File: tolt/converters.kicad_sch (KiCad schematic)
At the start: 60 parts, among them J11 Conn_01x05, U14 AMS1117-3.3, U15 LP5907MFX-3.3, U16 TPS62173DSG, U24 LTC7138xMSE, U25 LNK306D

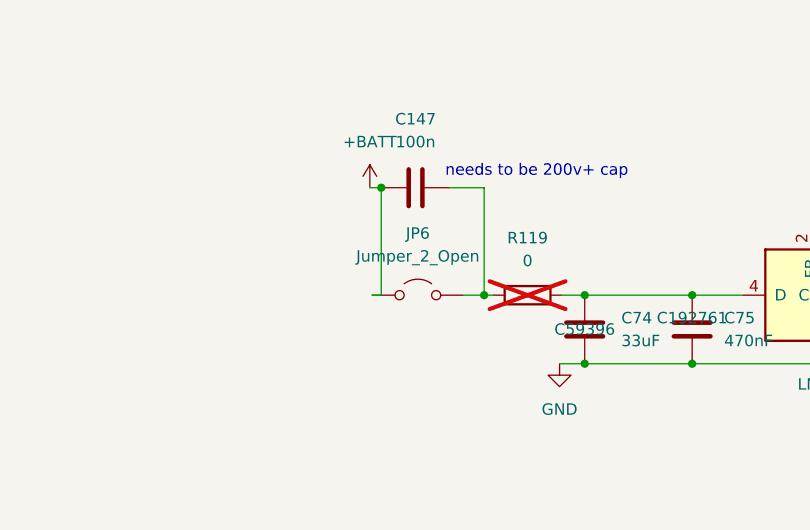
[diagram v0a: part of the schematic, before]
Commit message: 12vdc
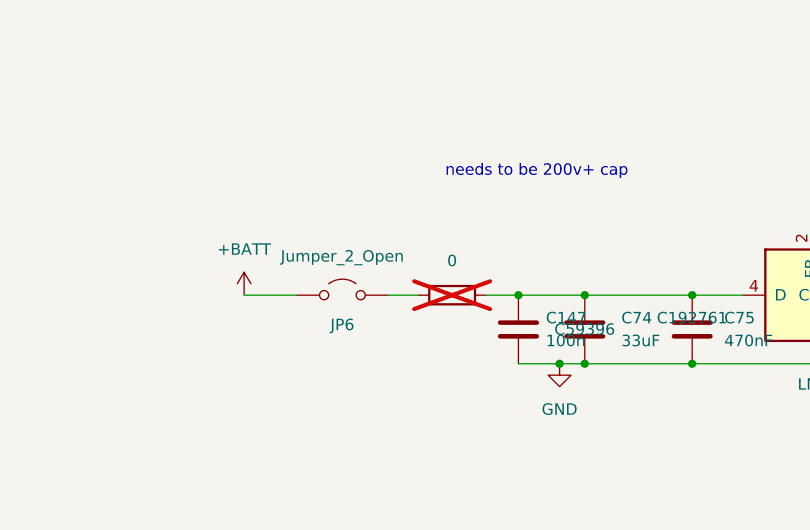
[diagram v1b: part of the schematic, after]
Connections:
- net +BATT: no longer C147.1
- net GND: now also C147.2
- net at JP6.2 (B), R119.1: no longer C147.2
- net at C74.1, C75.1, R119.2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: now also C147.1
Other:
- moved on the sheet: C147, JP6
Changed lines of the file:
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@@
 	)
 	(junction
-		(at 200.152 42.418)
+		(at 157.48 96.52)
 		(diameter 0)
 		(color 0 0 0 0)
 	)
 	(junction
-		(at 157.48 96.52)
+		(at 63.754 106.426)
 		(diameter 0)
 		(color 0 0 0 0)
 	)
 	(junction
-		(at 63.754 106.426)
+		(at 315.722 54.356)
 		(diameter 0)
 		(color 0 0 0 0)
 	)
 	(junction
-		(at 315.722 54.356)
+		(at 215.392 54.356)
 		(diameter 0)
 		(color 0 0 0 0)
@@
 	)
 	(junction
+		(at 219.964 61.976)
+		(diameter 0)
+		(color 0 0 0 0)
+	)
+	(junction
 		(at 338.328 199.644)
 		(diameter 0)
@@
 	)
 	(junction
-		(at 211.582 54.356)
-		(diameter 0)
-		(color 0 0 0 0)
-	)
-	(junction
 		(at 112.268 48.514)
 		(diameter 0)
@@
 	(wire
 		(pts
-			(xy 200.152 42.418) (xy 200.152 54.356)
-		)
-		(stroke
-			(width 0)
-			(type default)
-		)
-	)
-	(wire
-		(pts
 			(xy 169.926 96.52) (xy 179.07 96.52)
 		)
@@
 	(wire
 		(pts
-			(xy 211.582 54.356) (xy 212.598 54.356)
-		)
-		(stroke
-			(width 0)
-			(type default)
-		)
-	)
-	(wire
-		(pts
 			(xy 60.96 163.576) (xy 60.96 181.61)
 		)
@@
 	(wire
 		(pts
-			(xy 211.582 54.356) (xy 209.296 54.356)
-		)
-		(stroke
-			(width 0)
-			(type default)
-		)
-	)
-	(wire
-		(pts
-			(xy 200.152 54.356) (xy 199.136 54.356)
+			(xy 200.914 54.356) (xy 204.216 54.356)
 		)
 		(stroke
@@
 	(wire
 		(pts
-			(xy 220.218 54.356) (xy 222.758 54.356)
+			(xy 286.004 52.832) (xy 286.004 54.356)
 		)
 		(stroke
@@
 	(wire
 		(pts
-			(xy 286.004 52.832) (xy 286.004 54.356)
+			(xy 211.836 54.356) (xy 215.392 54.356)
 		)
 		(stroke
@@
 	(wire
 		(pts
-			(xy 198.882 42.418) (xy 200.152 42.418)
-		)
-		(stroke
-			(width 0)
-			(type default)
-		)
-	)
-	(wire
-		(pts
 			(xy 275.844 54.356) (xy 264.922 54.356)
 		)
@@
 	(wire
 		(pts
+			(xy 215.392 61.976) (xy 219.964 61.976)
+		)
+		(stroke
+			(width 0)
+			(type default)
+		)
+	)
+	(wire
+		(pts
 			(xy 160.274 161.036) (xy 148.844 161.036)
 		)
@@
 	(wire
 		(pts
-			(xy 207.772 42.418) (xy 211.582 42.418)
+			(xy 215.392 54.356) (xy 222.758 54.356)
 		)
 		(stroke
@@
 	(wire
 		(pts
-			(xy 211.582 42.418) (xy 211.582 54.356)
+			(xy 184.912 54.356) (xy 190.754 54.356)
 		)
 		(stroke
@@
 	(symbol
 		(lib_id "Device:R")
-		(at 216.408 54.356 90)
+		(at 208.026 54.356 90)
 		(unit 1)
 		(exclude_from_sim no)
@@
 		(on_board yes)
 		(dnp yes)
-		(fields_autoplaced yes)
 		(property "Reference" "R119"
-			(at 216.408 48.006 90)
+			(at 194.31 45.974 90)
 			(effects
 				(font
 					(size 1.27 1.27)
 				)
+				(hide yes)
 			)
 		)
 		(property "Value" "0"
-			(at 216.408 50.546 90)
+			(at 208.026 50.546 90)
 			(effects
 				(font
@@
 		)
 		(property "Footprint" "Resistor_SMD:R_0603_1608Metric"
-			(at 216.408 56.134 90)
+			(at 208.026 56.134 90)
 			(effects
 				(font
@@
 		)
 		(property "Datasheet" "~"
-			(at 216.408 54.356 0)
+			(at 208.026 54.356 0)
 			(effects
 				(font
@@
 		)
 		(property "Description" "Resistor"
-			(at 216.408 54.356 0)
+			(at 208.026 54.356 0)
 			(effects
 				(font
@@
 		)
 		(property "Availability" ""
-			(at 216.408 54.356 0)
+			(at 208.026 54.356 0)
 			(effects
 				(font
@@
 		)
 		(property "Check_prices" ""
-			(at 216.408 54.356 0)
+			(at 208.026 54.356 0)
 			(effects
 				(font
@@
 		)
 		(property "Description_1" ""
-			(at 216.408 54.356 0)
+			(at 208.026 54.356 0)
 			(effects
 				(font
@@
 		)
 		(property "MANUFACTURER" ""
-			(at 216.408 54.356 0)
+			(at 208.026 54.356 0)
 			(effects
 				(font
@@
 		)
 		(property "MAXIMUM_PACKAGE_HEIGHT" ""
-			(at 216.408 54.356 0)
+			(at 208.026 54.356 0)
 			(effects
 				(font
@@
 		)
 		(property "MF" ""
-			(at 216.408 54.356 0)
+			(at 208.026 54.356 0)
 			(effects
 				(font
@@
 		)
 		(property "MFR PT" ""
-			(at 216.408 54.356 0)
+			(at 208.026 54.356 0)
 			(effects
 				(font
@@
 		)
 		(property "MP" ""
-			(at 216.408 54.356 0)
+			(at 208.026 54.356 0)
 			(effects
 				(font
@@
 		)
 		(property "PARTREV" ""
-			(at 216.408 54.356 0)
+			(at 208.026 54.356 0)
 			(effects
 				(font
@@
 		)
 		(property "Package" ""
-			(at 216.408 54.356 0)
+			(at 208.026 54.356 0)
 			(effects
 				(font
@@
 		)
 		(property "Price" ""
-			(at 216.408 54.356 0)
+			(at 208.026 54.356 0)
 			(effects
 				(font
@@
 		)
 		(property "STANDARD" ""
-			(at 216.408 54.356 0)
+			(at 208.026 54.356 0)
 			(effects
 				(font
@@
 		)
 		(property "SnapEDA_Link" ""
-			(at 216.408 54.356 0)
+			(at 208.026 54.356 0)
 			(effects
 				(font
@@
 	(symbol
 		(lib_id "power:+BATT")
-		(at 198.882 42.418 0)
+		(at 184.912 54.356 0)
 		(unit 1)
 		(exclude_from_sim no)
@@
 		(fields_autoplaced yes)
 		(property "Reference" "#PWR0164"
-			(at 198.882 46.228 0)
+			(at 184.912 58.166 0)
 			(effects
 				(font
@@
 		)
 		(property "Value" "+BATT"
-			(at 198.882 37.338 0)
+			(at 184.912 49.276 0)
 			(effects
 				(font
@@
 		)
 		(property "Footprint" ""
-			(at 198.882 42.418 0)
+			(at 184.912 54.356 0)
 			(effects
 				(font
@@
 		)
 		(property "Datasheet" ""
-			(at 198.882 42.418 0)
+			(at 184.912 54.356 0)
 			(effects
 				(font
@@
 		)
 		(property "Description" "Power symbol creates a global label with name \"+BATT\""
-			(at 198.882 42.418 0)
+			(at 184.912 54.356 0)
 			(effects
 				(font
@@
 	(symbol
 		(lib_id "Device:C")
-		(at 203.962 42.418 90)
+		(at 215.392 58.166 0)
 		(unit 1)
 		(exclude_from_sim no)
@@
 		(fields_autoplaced yes)
 		(property "Reference" "C147"
-			(at 203.962 34.798 90)
+			(at 218.44 56.8959 0)
 			(effects
 				(font
 					(size 1.27 1.27)
 				)
+				(justify left)
 			)
 		)
 		(property "Value" "100n"
-			(at 203.962 37.338 90)
+			(at 218.44 59.4359 0)
 			(effects
 				(font
 					(size 1.27 1.27)
 				)
+				(justify left)
 			)
 		)
 		(property "Footprint" "Capacitor_SMD:C_1210_3225Metric"
-			(at 207.772 41.4528 0)
+			(at 216.3572 61.976 0)
 			(effects
 				(font
@@
 		)
 		(property "Datasheet" "~"
-			(at 203.962 42.418 0)
+			(at 215.392 58.166 0)
 			(effects
 				(font
@@
 		)
 		(property "Description" "Unpolarized capacitor"
-			(at 203.962 42.418 0)
+			(at 215.392 58.166 0)
 			(effects
 				(font
@@
 	(symbol
 		(lib_id "Jumper:Jumper_2_Open")
-		(at 204.216 54.356 0)
+		(at 195.834 54.356 0)
 		(unit 1)
 		(exclude_from_sim yes)
@@
 		(on_board yes)
 		(dnp no)
-		(fields_autoplaced yes)
 		(property "Reference" "JP6"
-			(at 204.216 47.498 0)
+			(at 195.834 57.658 0)
 			(effects
 				(font
@@
 		)
 		(property "Value" "Jumper_2_Open"
-			(at 204.216 50.038 0)
+			(at 195.834 50.038 0)
 			(effects
 				(font
@@
 		)
 		(property "Footprint" "Connector_PinHeader_2.54mm:PinHeader_1x02_P2.54mm_Vertical"
-			(at 204.216 54.356 0)
+			(at 195.834 54.356 0)
 			(effects
 				(font
@@
 		)
 		(property "Datasheet" "~"
-			(at 204.216 54.356 0)
+			(at 195.834 54.356 0)
 			(effects
 				(font
@@
 		)
 		(property "Description" "Jumper, 2-pole, open"
-			(at 204.216 54.356 0)
+			(at 195.834 54.356 0)
 			(effects
 				(font

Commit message: begenning of lcsc part assign
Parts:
- C102, C105: footprint Capacitor_SMD:C_2220_5750Metric_Pad1.97x5.40mm_HandSolder -> Capacitor_SMD:C_2220_5750Metric
- C149, C71, C73, C85: LCSC (none) -> C138687
- C150: footprint Capacitor_SMD:C_1206_3216Metric_Pad1.33x1.80mm_HandSolder -> Capacitor_SMD:C_1206_3216Metric
- C66: LCSC (none) -> C15008
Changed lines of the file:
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@@
 			)
 		)
+		(property "LCSC" "C138687"
+			(at 170.942 164.846 0)
+			(effects
+				(font
+					(size 1.27 1.27)
+				)
+				(hide yes)
+			)
+		)
 		(pin "1"
 		)
@@
 			)
 		)
+		(property "LCSC" "C138687"
+			(at 112.268 44.704 0)
+			(effects
+				(font
+					(size 1.27 1.27)
+				)
+				(hide yes)
+			)
+		)
 		(pin "1"
 		)
@@
 			)
 		)
+		(property "LCSC" "C138687"
+			(at 148.844 164.846 0)
+			(effects
+				(font
+					(size 1.27 1.27)
+				)
+				(hide yes)
+			)
+		)
 		(pin "1"
 		)
@@
 			)
 		)
+		(property "LCSC" "C138687"
+			(at 47.752 43.688 0)
+			(effects
+				(font
+					(size 1.27 1.27)
+				)
+				(hide yes)
+			)
+		)
 		(pin "1"
 		)
@@
 			)
 		)
-		(property "Footprint" "Capacitor_SMD:C_2220_5750Metric_Pad1.97x5.40mm_HandSolder"
+		(property "Footprint" "Capacitor_SMD:C_2220_5750Metric"
 			(at 20.0152 177.8 0)
 			(effects
@@
 			)
 		)
-		(property "Footprint" "Capacitor_SMD:C_2220_5750Metric_Pad1.97x5.40mm_HandSolder"
+		(property "Footprint" "Capacitor_SMD:C_2220_5750Metric"
 			(at 31.4452 177.8 0)
 			(effects
@@
 			)
 		)
-		(property "Footprint" "Capacitor_SMD:C_1206_3216Metric_Pad1.33x1.80mm_HandSolder"
+		(property "Footprint" "Capacitor_SMD:C_1206_3216Metric"
 			(at 265.8872 54.356 0)
 			(effects
@@
 			(at 222.758 100.33 0)
 			(effects
+				(font
+					(size 1.27 1.27)
+				)
+				(hide yes)
+			)
+		)
+		(property "LCSC" "C15008"
+			(at 222.758 100.33 0)
+			(effects
